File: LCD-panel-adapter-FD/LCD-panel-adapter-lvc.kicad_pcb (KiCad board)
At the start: 2 copper layers, 40.6 x 48.3 mm, 13 parts, among them J101 HEADER_18, M101 LOGO_OSHW, P101 CONN_4X2, P102 CONN_5X2, P103 CONN_5X2, U101 74HC07A

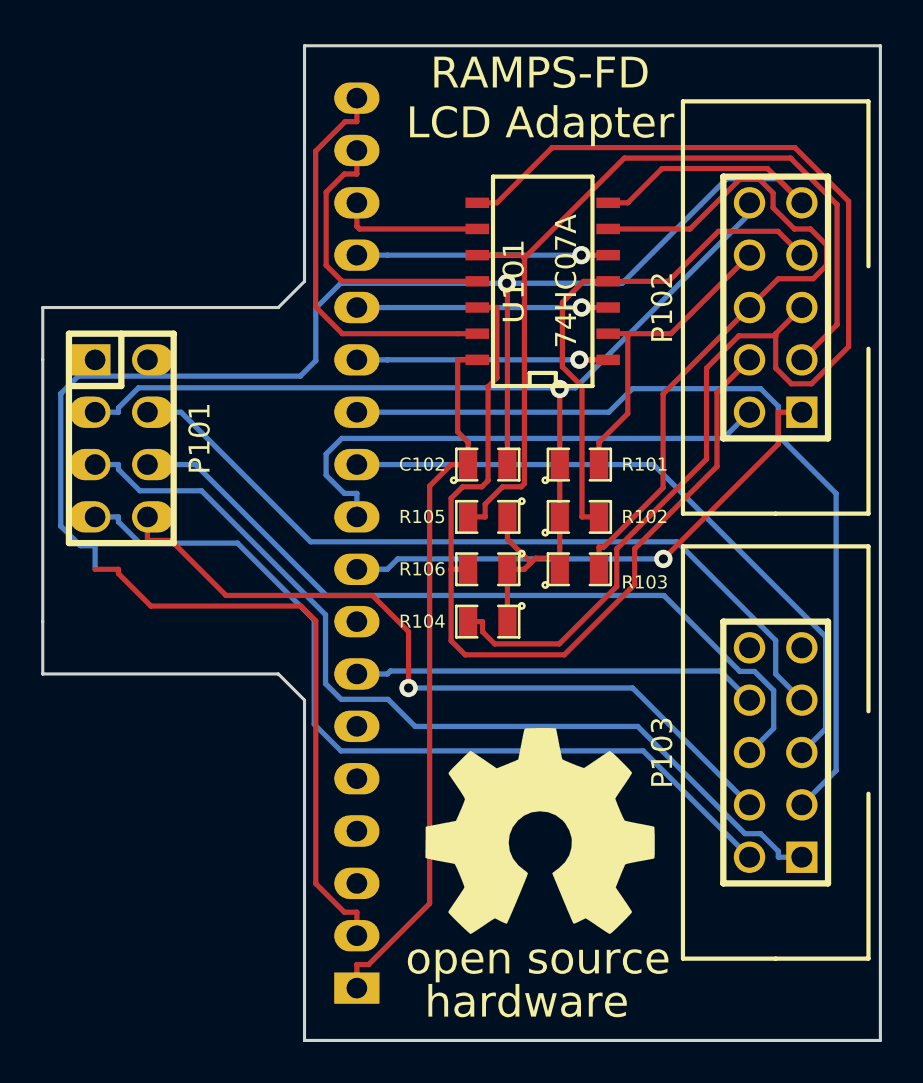
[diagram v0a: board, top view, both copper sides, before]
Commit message: LCD-Panel-adapter: routing, gerbers
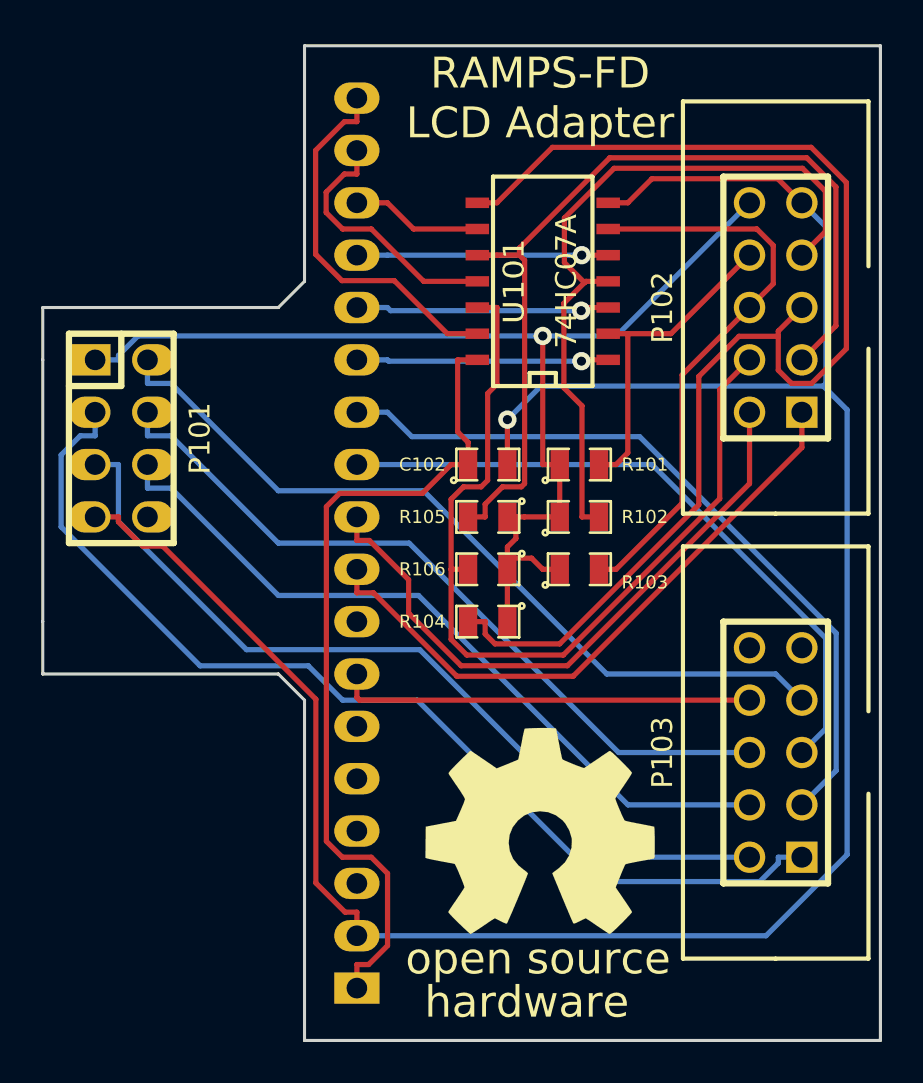
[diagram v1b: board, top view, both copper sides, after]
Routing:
- net GND: track 99.8 -> 113.8 mm
- net /LCD_D6_5V: track 25.2 -> 35.4 mm
- net /LCD_D5_5V: track 34.8 -> 28.0 mm
- net /SD_DO: track 44.4 -> 50.4 mm
- net /ENC2: track 42.5 -> 36.7 mm
- net /IOREF: track 34.7 -> 40.3 mm
- net /ENC_SW: track 25.4 -> 30.8 mm
- net /BEEP: track 25.6 -> 30.7 mm, vias 1 -> 0
- net +5V: track 53.2 -> 55.2 mm
- net /SD_DI: track 38.4 -> 36.7 mm
- net /LCD_E: track 14.2 -> 12.7 mm
- net /LCD_RS: track 19.7 -> 18.2 mm
- net /LCD_E_5V: track 43.4 -> 44.2 mm
- net /SD_DETECT: track 38.5 -> 39.3 mm
- net /LCD_D4: track 7.04 -> 6.37 mm
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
